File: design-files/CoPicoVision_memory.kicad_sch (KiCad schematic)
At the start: 9 parts, among them U103 74ACT05, U201 GAL22V10, U202 GAL22V10, U203 AT28C64, U204 AS6C6264

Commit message: All the bypass caps are now 0805s.
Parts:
- C201, C202, C203, C204: footprint Capacitor_THT:C_Disc_D3.8mm_W2.6mm_P2.50mm -> Capacitor_SMD:C_0805_2012Metric_Pad1.18x1.45mm_HandSolder
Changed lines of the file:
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@@
       (effects (font (size 1.27 1.27)) (justify left))
     )
-    (property "Footprint" "Capacitor_THT:C_Disc_D3.8mm_W2.6mm_P2.50mm" (at 110.871 158.496 0)
+    (property "Footprint" "Capacitor_SMD:C_0805_2012Metric_Pad1.18x1.45mm_HandSolder" (at 110.871 158.496 0)
       (effects (font (size 1.27 1.27)) hide)
     )
@@
       (effects (font (size 1.27 1.27)) (justify left))
     )
-    (property "Footprint" "Capacitor_THT:C_Disc_D3.8mm_W2.6mm_P2.50mm" (at 87.884 158.496 0)
+    (property "Footprint" "Capacitor_SMD:C_0805_2012Metric_Pad1.18x1.45mm_HandSolder" (at 87.884 158.496 0)
       (effects (font (size 1.27 1.27)) hide)
     )
@@
       (effects (font (size 1.27 1.27)) (justify left))
     )
-    (property "Footprint" "Capacitor_THT:C_Disc_D3.8mm_W2.6mm_P2.50mm" (at 76.454 158.496 0)
+    (property "Footprint" "Capacitor_SMD:C_0805_2012Metric_Pad1.18x1.45mm_HandSolder" (at 76.454 158.496 0)
       (effects (font (size 1.27 1.27)) hide)
     )
@@
       (effects (font (size 1.27 1.27)) (justify left))
     )
-    (property "Footprint" "Capacitor_THT:C_Disc_D3.8mm_W2.6mm_P2.50mm" (at 99.441 158.496 0)
+    (property "Footprint" "Capacitor_SMD:C_0805_2012Metric_Pad1.18x1.45mm_HandSolder" (at 99.441 158.496 0)
       (effects (font (size 1.27 1.27)) hide)
     )

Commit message: Controller section is mostly SMT now.
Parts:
- U103: footprint Package_DIP:DIP-14_W7.62mm_Socket -> Package_SO:SOIC-14_3.9x8.7mm_P1.27mm
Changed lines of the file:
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@@
       (effects (font (size 1.27 1.27)))
     )
-    (property "Footprint" "Package_DIP:DIP-14_W7.62mm_Socket" (at 143.129 106.299 0)
+    (property "Footprint" "Package_SO:SOIC-14_3.9x8.7mm_P1.27mm" (at 143.129 106.299 0)
       (effects (font (size 1.27 1.27)) hide)
     )

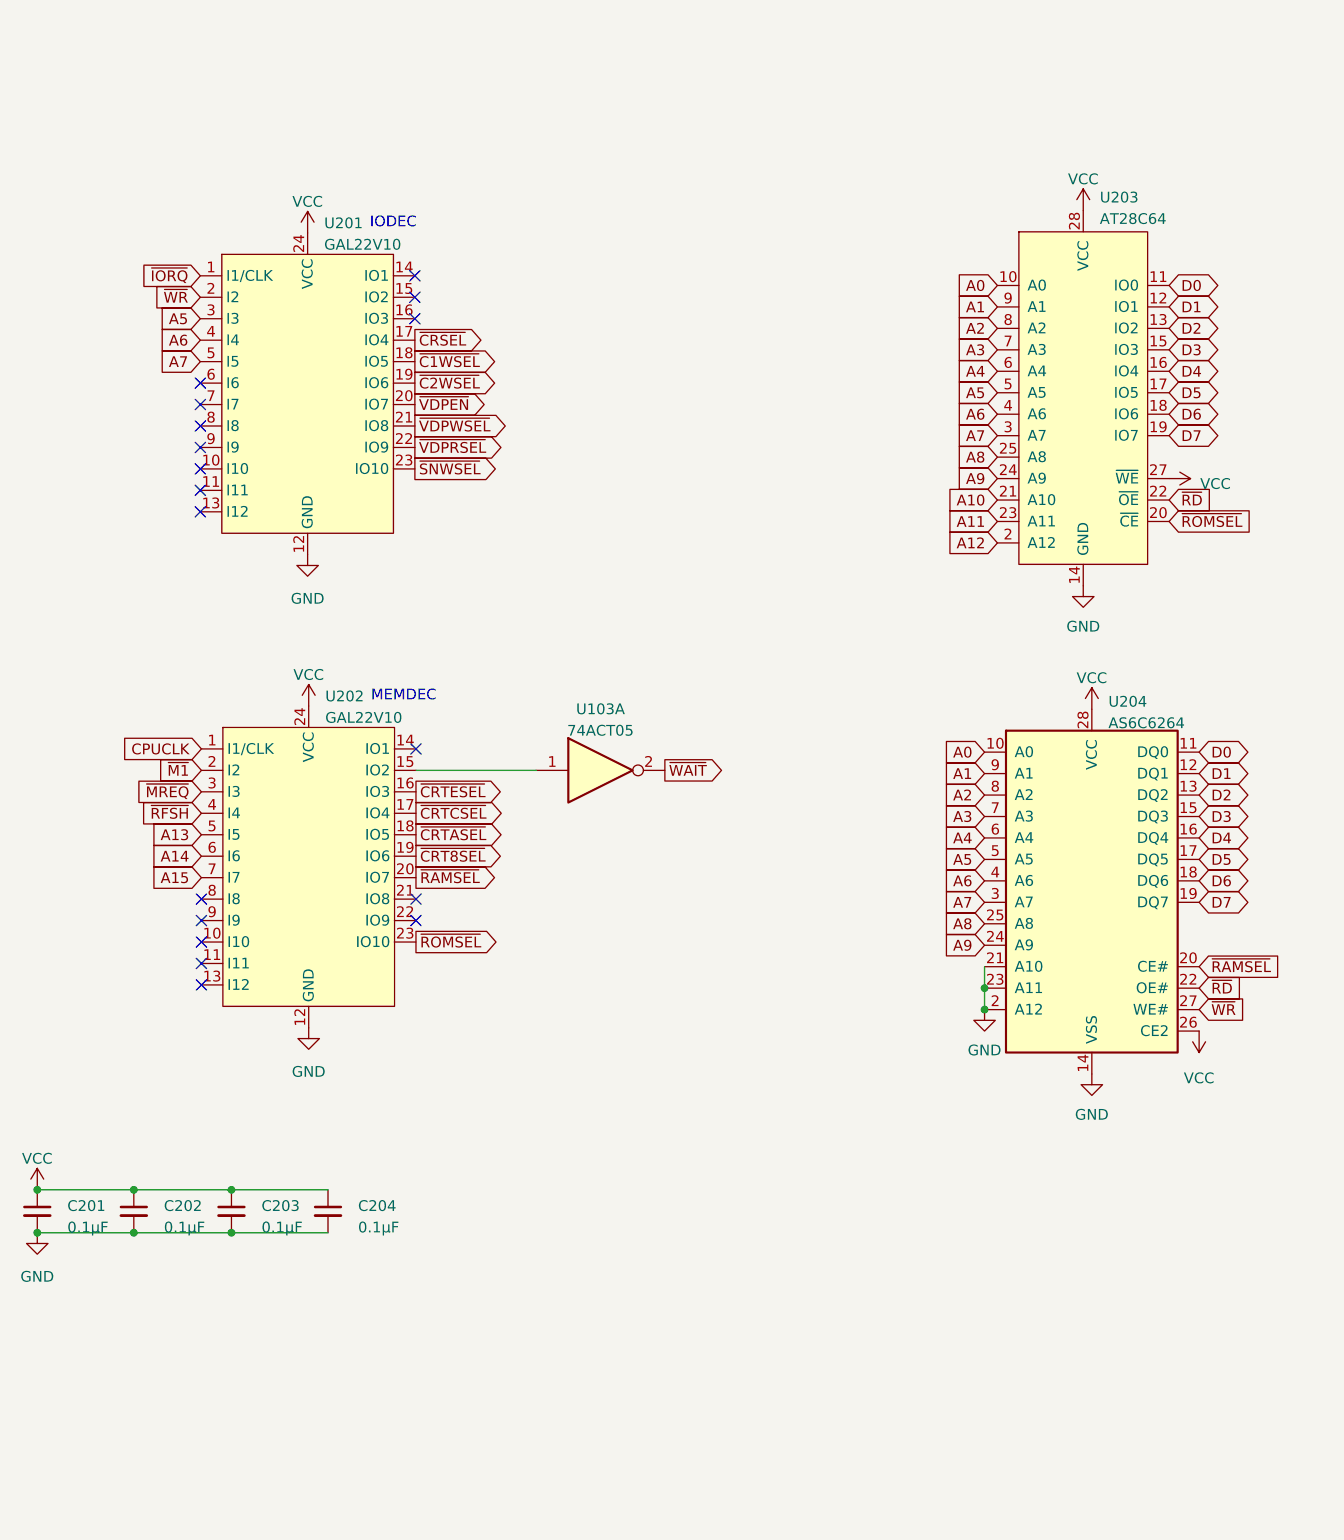
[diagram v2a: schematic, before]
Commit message: Add the SGM memory logic chips, clean out board routing on the left half of the board.
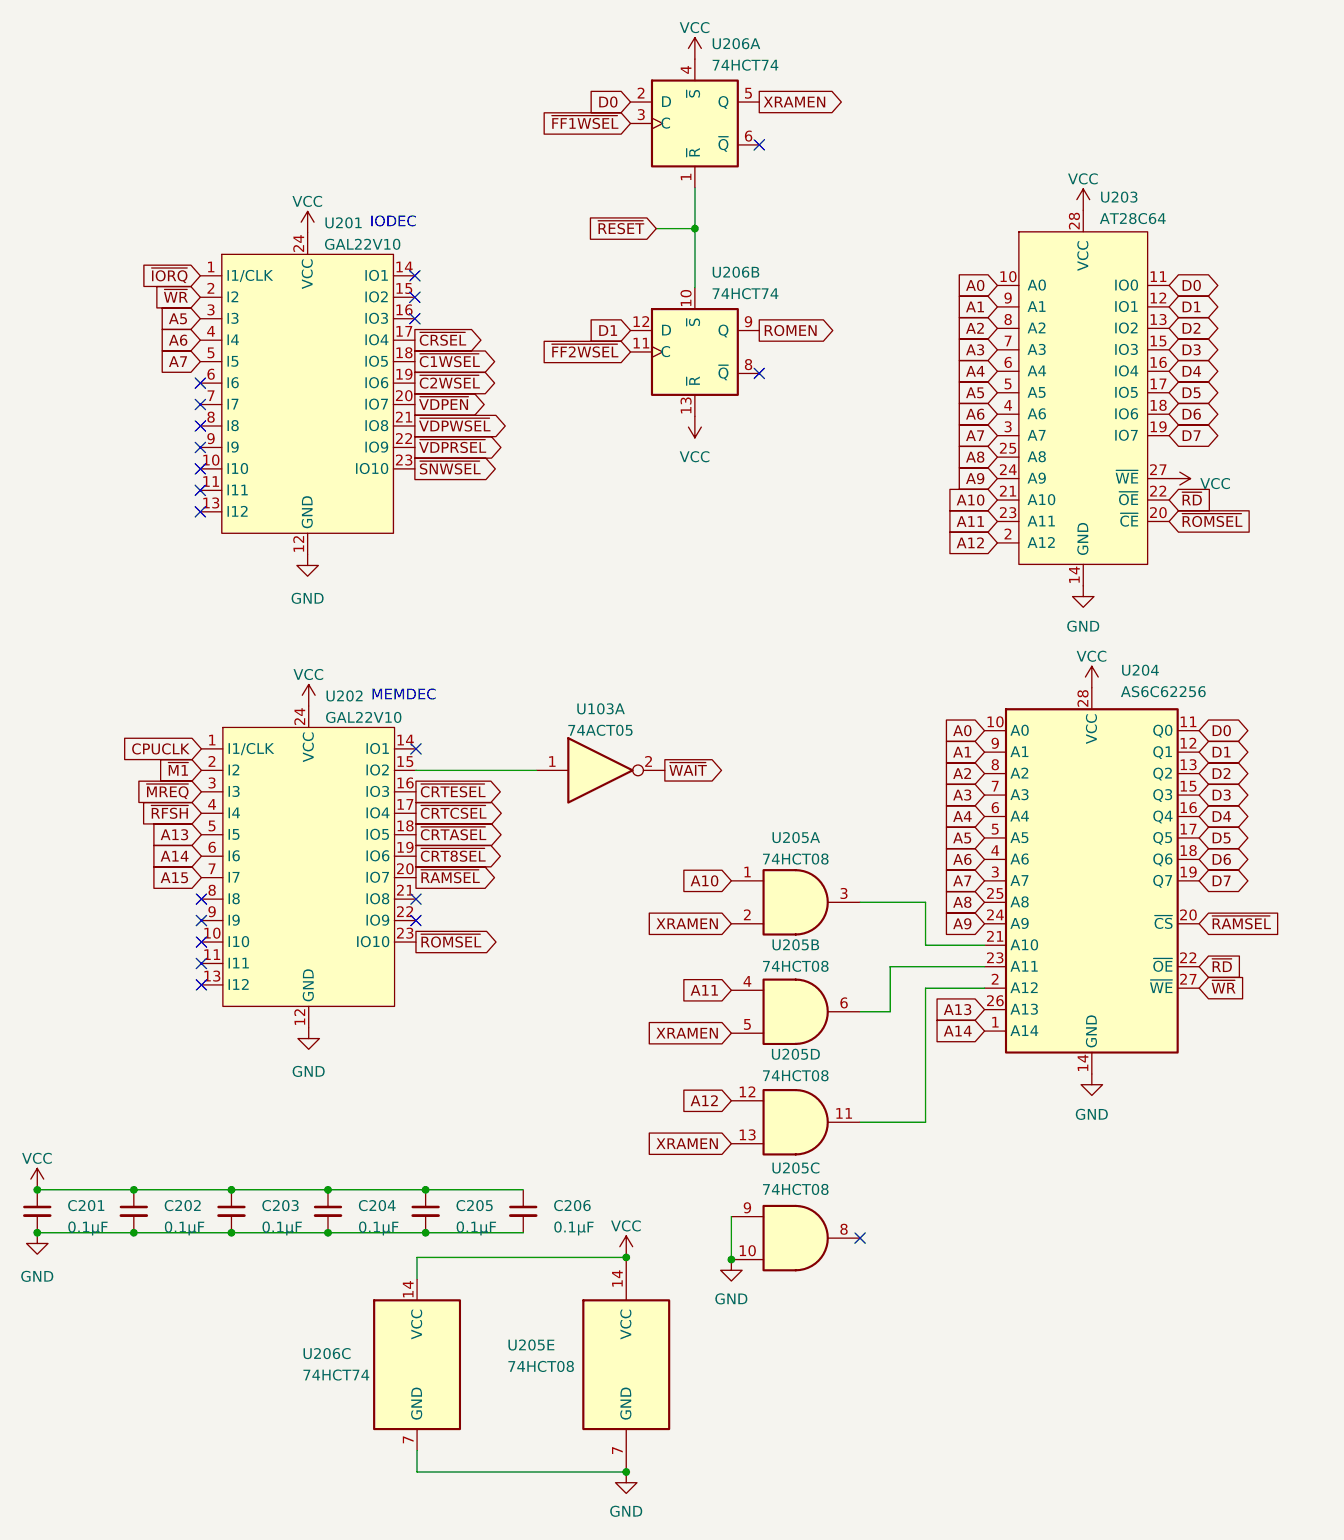
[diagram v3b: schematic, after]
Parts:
- added C205, C206: 0.1µF, Capacitor_SMD:C_0805_2012Metric_Pad1.18x1.45mm_HandSolder, symbol Device:C_Small
- added U205: 74HCT08, Package_SO:SOIC-14_3.9x8.7mm_P1.27mm, symbol 74xx:74LS08
- added U206: 74HCT74, Package_SO:SOIC-14_3.9x8.7mm_P1.27mm, symbol 74xx:74HC74
- U204: value AS6C6264 -> AS6C62256; footprint Package_DIP:DIP-28_W15.24mm_Socket -> Package_SO:SOIC-28W_7.5x17.9mm_P1.27mm; symbol jrt-ICs:AS6C6264 -> Memory_RAM:CY62256-70PC
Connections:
- net A10: now also U205.1
- net A11: now also U205.4
- net A12: now also U205.12
- net A13: now also U204.26 (A13)
- net A14: now also U204.1 (A14)
- net D0: now also U206.2 (D)
- net D1: now also U206.12 (D)
- net GND: now also C205.2, C206.2, U205.10, U205.7 (GND), U205.9, U206.7 (GND); no longer U204.2 (A12), U204.21 (A10), U204.23 (A11)
- net VCC: now also C205.1, C206.1, U205.14 (VCC), U206.13 (~{R}), U206.14 (VCC), U206.4 (~{S}); no longer U204.26 (CE2)
- new net: U204.21 (A10), U205.3
- new net: U204.2 (A12), U205.11
- new net: U204.23 (A11), U205.6
- new net ROMEN: U206.9 (Q)
- new net XRAMEN: U205.13, U205.2, U205.5, U206.5 (Q)
- new net ~{FF1WSEL}: U206.3 (C)
- new net ~{FF2WSEL}: U206.11 (C)
- new net ~{RESET}: U206.1 (~{R}), U206.10 (~{S})
- no-connect marks 18 -> 21

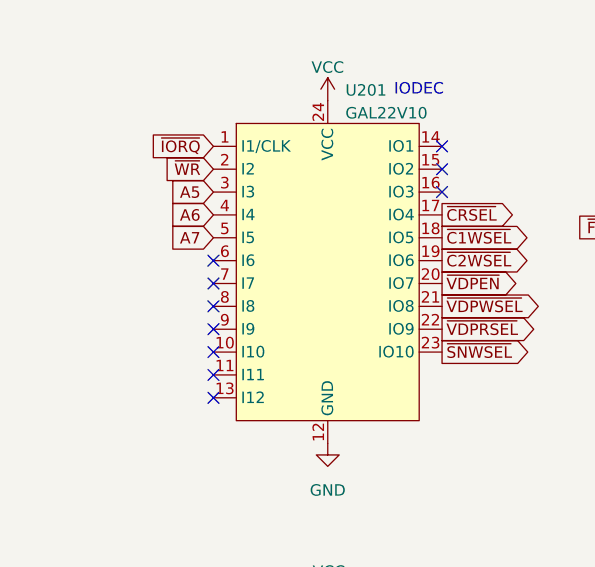
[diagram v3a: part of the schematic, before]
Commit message: Re-pin the inputs of the IODEC GAL, and make it take A0-A7 in prep for SGM additions.
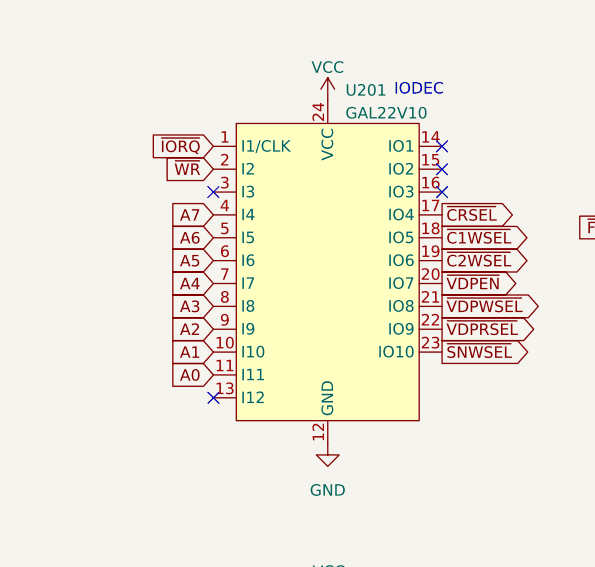
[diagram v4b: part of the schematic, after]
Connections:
- net A0: now also U201.11 (I11)
- net A1: now also U201.10 (I10)
- net A2: now also U201.9 (I9)
- net A3: now also U201.8 (I8)
- net A4: now also U201.7 (I7)
- net A5: now also U201.6 (I6); no longer U201.3 (I3)
- net A6: now also U201.5 (I5); no longer U201.4 (I4)
- net A7: now also U201.4 (I4); no longer U201.5 (I5)
- no-connect marks 21 -> 16
